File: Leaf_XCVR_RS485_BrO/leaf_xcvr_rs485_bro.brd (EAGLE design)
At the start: 23 x 45.4 mm, 14 parts, among them J1 CONN_6X1_JST_PA, J2 CONN_4X1_JST_PA, U1 RS485_XCVR_SN65HVD178X

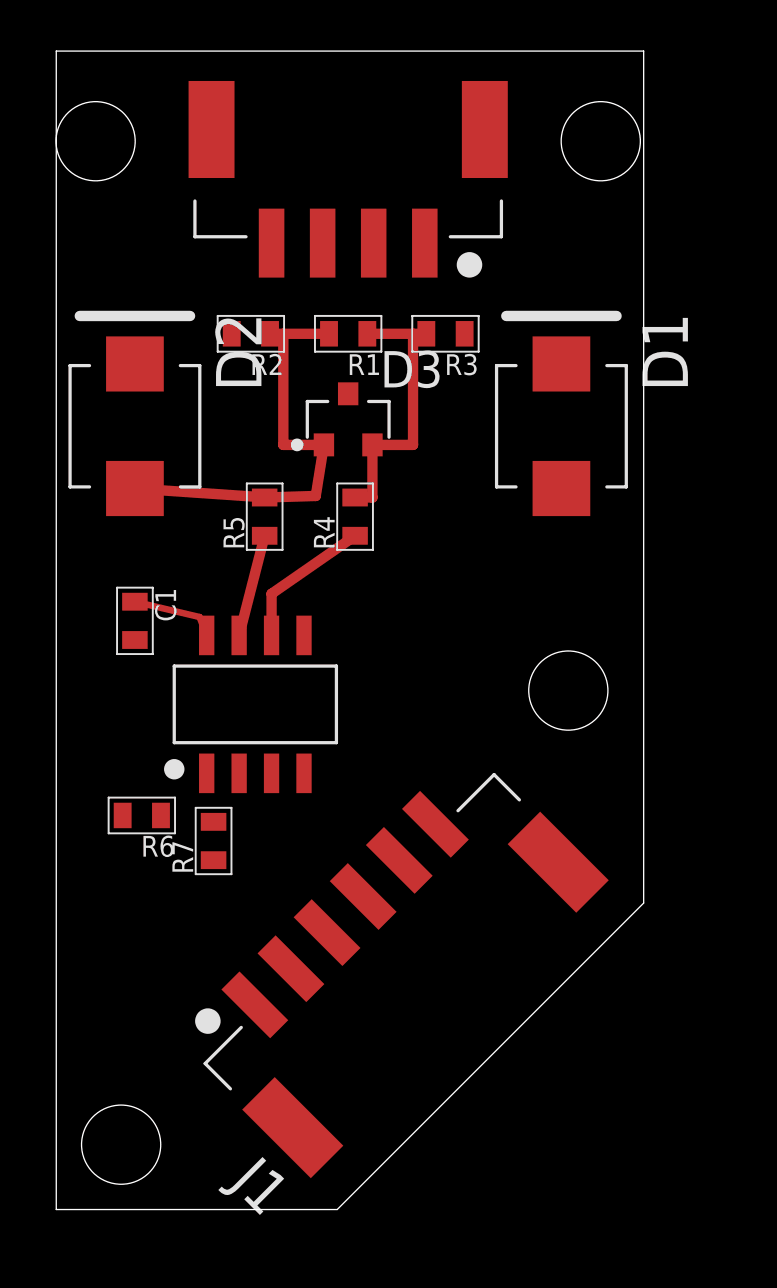
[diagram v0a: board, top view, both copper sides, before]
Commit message: latest and greatest
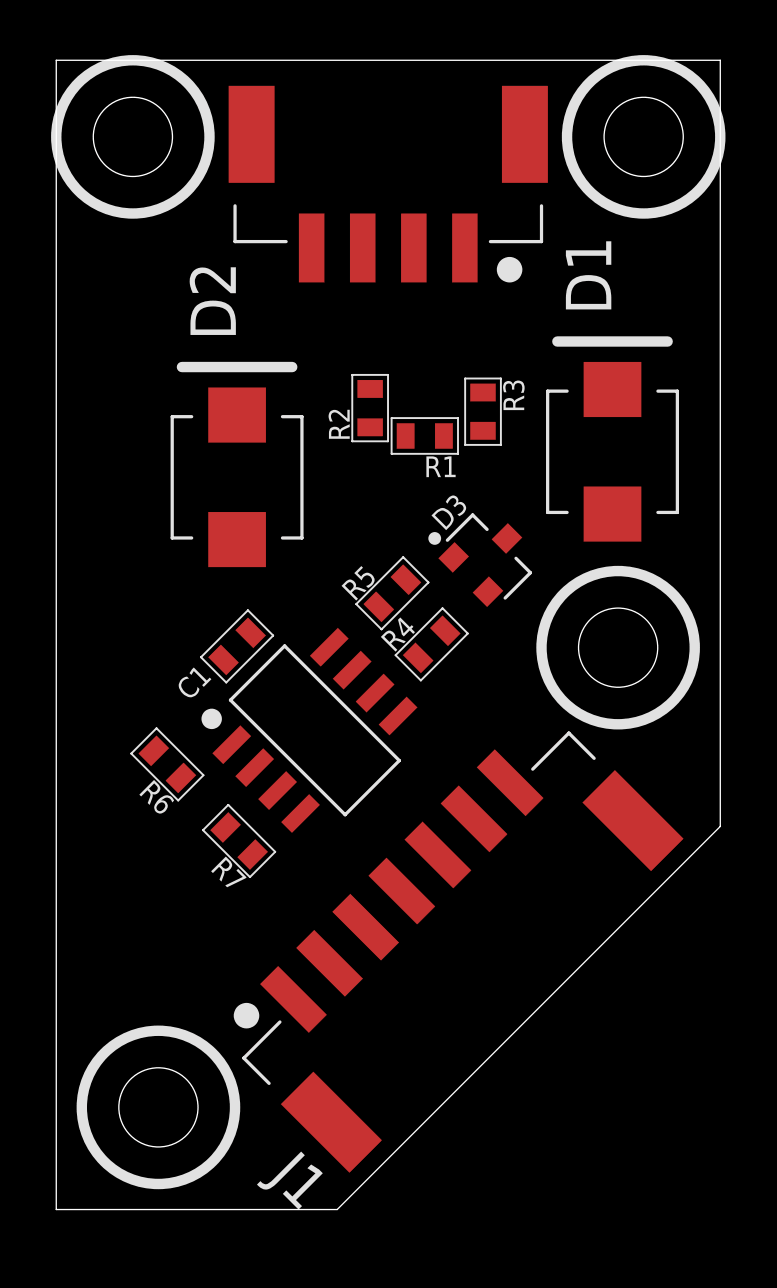
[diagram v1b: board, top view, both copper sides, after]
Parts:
- J1: value CONN_6X1_JST_PA -> CONN_7X1_JST_PA; device leaf:CONN_6X1_JST_PA -> leaf:CONN_7X1_JST_PA
- moved D3 7.69 mm to (16.9, 25.6), turned to 315 degrees
- moved R4 5.83 mm to (14.7, 22.1), turned to 45 degrees
- moved R5 5.83 mm to (13.2, 24.1), turned to 45 degrees
- moved R2 5.50 mm to (12.3, 31.4), turned to 90 degrees
- moved R1 5.00 mm to (14.4, 30.3)
- moved D2 4.47 mm to (7.08, 28.7)
- moved C1 4.12 mm to (7.08, 22.1), turned to 225 degrees
- moved R3 3.39 mm to (16.7, 31.2), turned to 270 degrees
- moved U1 2.91 mm to (8.78, 20.1), turned to 315 degrees
- moved J1 2.40 mm to (20.0, 6.00)
- moved D1 2.24 mm to (21.8, 29.7)
- moved R6 2.24 mm to (4.35, 17.4), turned to 135 degrees
- moved J2 1.58 mm to (13.0, 46.8)
- moved R7 1.00 mm to (7.16, 14.4), turned to 135 degrees
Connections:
- removed net GND: C1.P$2, D1.P$1, D2.P$1, D3.3, J1.1, J2.1, R3.P$1, R7.P$1, U1.5
- removed net N$4: J1.2
- removed net N$5: J2.4
- new net GND1: C1.P$2, D1.P$1, D2.P$1, D3.3, J1.3, R3.P$1, R7.P$1, U1.5
- new net GND2: J1.1, J2.1
- new net V+: J1.2, J2.4
- net +3V3: now also J1.4; no longer J1.3
- net N$10: now also J1.7; no longer J1.6
- net N$8: now also J1.6; no longer J1.5
- net N$9: now also J1.5; no longer J1.4
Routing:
- net N$7: track 17.5 -> 0.00 mm
- net N$6: track 11.0 -> 0.00 mm
- net N$1: track 5.61 -> 0.00 mm
- net N$2: track 4.03 -> 0.00 mm
- net +3V3: track 3.37 -> 0.00 mm
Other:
- board size 23 x 45.4 mm -> 26 x 45 mm

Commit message: submission to OSHpark
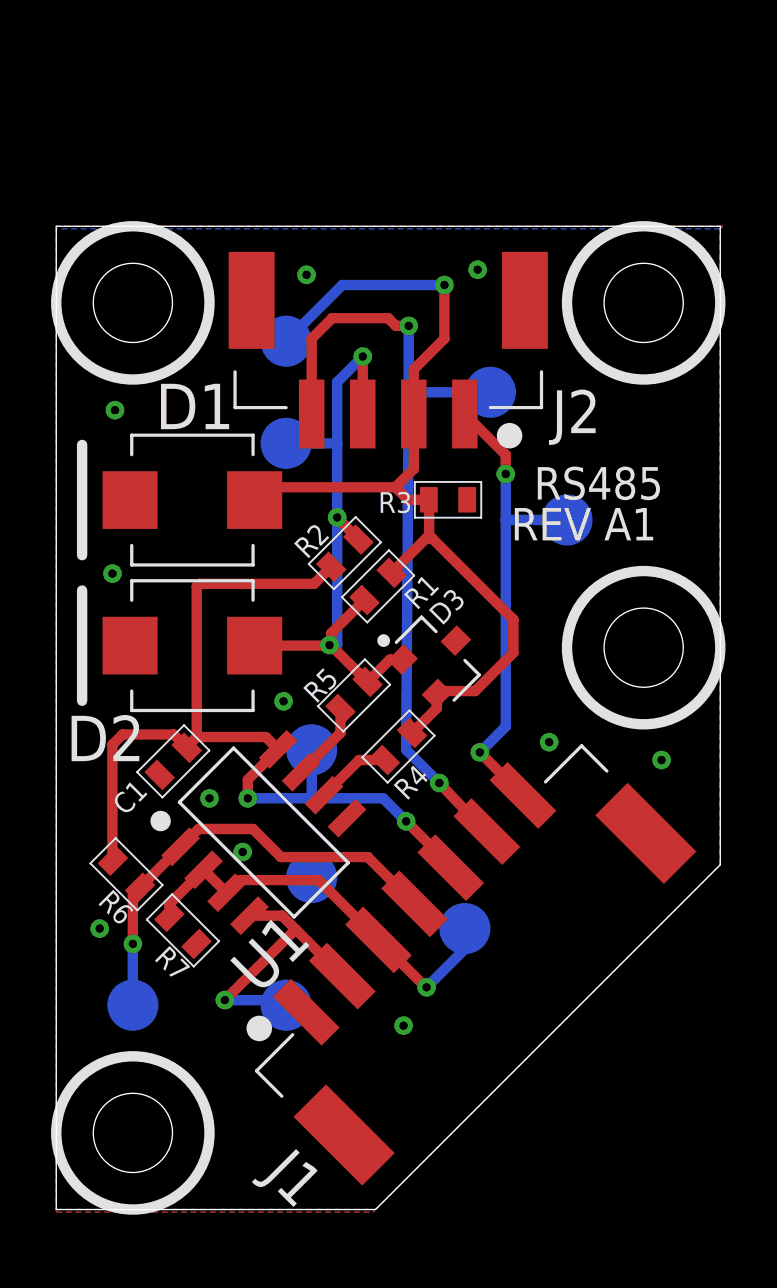
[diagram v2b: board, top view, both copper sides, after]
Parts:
- added TP1, TP2, TP3, TP4, TP5, TP6, TP7, TP8, TP9: TP1, leaf:TP1
- added U$1: STEPS_LOGO, stepOSP:STEPS_LOGO
- C1: value (none) -> 0.1u
- R1: value (none) -> 120
- R4, R5: value (none) -> 10
- R6, R7: value (none) -> 3.3k
- moved D1 16.6 mm to (5.33, 27.8), turned to 0 degrees
- moved D2 6.82 mm to (5.33, 22.1), turned to 0 degrees
- moved J2 6.50 mm to (13.0, 40.3)
- moved R1 6.17 mm to (12.6, 24.4), turned to 225 degrees
- moved R2 5.77 mm to (11.3, 25.7), turned to 225 degrees
- moved C1 5.15 mm to (4.58, 17.6)
- moved R6 4.59 mm to (2.75, 13.1)
- moved D3 4.47 mm to (14.9, 21.6)
- moved U1 4.47 mm to (6.78, 16.1)
- moved R5 4.27 mm to (11.7, 20.1)
- moved R4 4.21 mm to (13.4, 18.1)
- moved R7 4.13 mm to (4.96, 10.9)
- moved R3 3.71 mm to (15.3, 27.8), turned to 180 degrees
- moved J1 0.71 mm to (20.5, 5.50)
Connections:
- net +3V3: now also J1.5, TP6.P$1; no longer J1.4
- net GND1: now also D1.1, D2.1, J1.1, TP9.P$1; no longer D1.P$1, D2.P$1, J1.3
- net GND2: now also J1.7, TP8.P$1; no longer J1.1
- net N$10: now also J1.2, TP3.P$1; no longer J1.7
- net N$6: now also D1.2, TP2.P$1; no longer D1.P$2
- net N$7: now also D2.2, TP1.P$1; no longer D2.P$2
- net N$8: now also J1.3, TP5.P$1; no longer J1.6
- net N$9: now also J1.4, TP4.P$1; no longer J1.5
- net V+: now also J1.6, TP7.P$1; no longer J1.2
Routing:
- net N$6: track 0.00 -> 39.1 mm, vias 0 -> 1
- net +3V3: track 0.00 -> 36.9 mm, vias 0 -> 2
- net V+: track 0.00 -> 31.5 mm, vias 0 -> 2
- net N$7: track 0.00 -> 26.6 mm, vias 0 -> 3
- net GND2: track 0.00 -> 19.1 mm, vias 0 -> 2
- net N$9: track 0.00 -> 17.6 mm, vias 0 -> 1
- net N$8: track 0.00 -> 16.4 mm, vias 0 -> 1
- net N$10: track 0.00 -> 11.0 mm, vias 0 -> 1
- net N$2: track 0.00 -> 3.12 mm
- net N$1: track 0.00 -> 2.95 mm
- added copper zone on layer 1, net GND1
- added copper zone on layer 16, net GND1
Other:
- board size 26 x 45 mm -> 26 x 38.5 mm
- board text added: "Project Leaf"
- board text added: "REV A1"
- board text added: "RS485"
